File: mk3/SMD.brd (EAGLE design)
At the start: 31.3 x 39 mm, 13 parts, among them IC1 744053D

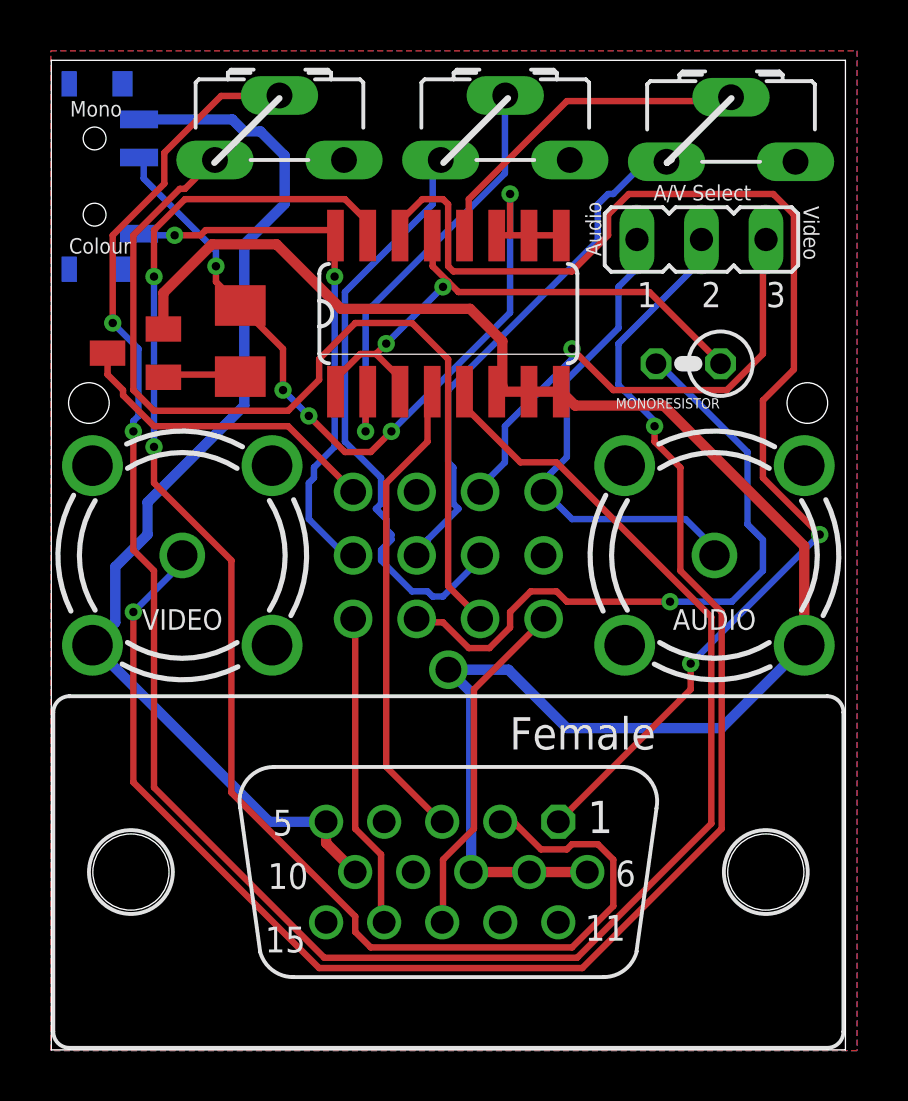
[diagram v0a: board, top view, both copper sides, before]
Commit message: CD4053
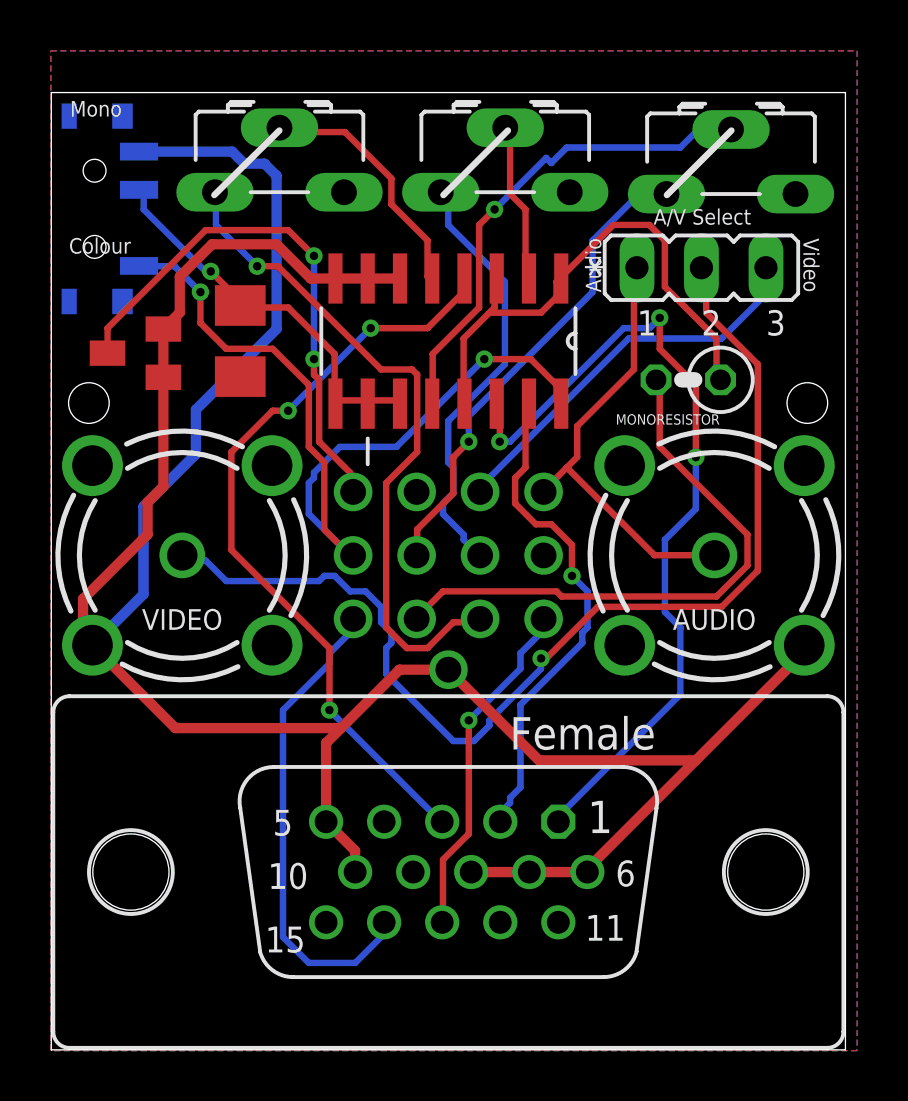
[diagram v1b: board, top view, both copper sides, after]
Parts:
- removed IC1: 744053D, 74xx-eu:SO16
- added U1: CD4053BCM, Fairchild_By_element14_Batch_1:SOIC127P600X175-16N
- moved R7 1.27 mm to (26.8, 33.7)
- moved R8 1.27 mm to (17.9, 33.8)
- moved R9 1.27 mm to (9.00, 33.8)
- moved S1 1.27 mm to (1.72, 33.1)
- moved JP1 1.11 mm to (25.6, 30.8)
- moved MONORESISTOR 0.64 mm to (25.1, 26.4)
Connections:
- removed net N$6: IC1.5, R9.S
- new net N$2: R7.S, U1.12
- net GND: now also U1.6, U1.7, U1.8; no longer IC1.6, IC1.7, IC1.8
- net MONOSIGNAL: now also U1.1, U1.13, U1.3; no longer IC1.1, IC1.13, IC1.3
- net N$4: now also R8.S, U1.2; no longer IC1.12, R7.S
- net N$5: now also R9.S, U1.5; no longer IC1.2, R8.S
- net SELECT: now also U1.10, U1.11, U1.9; no longer IC1.10, IC1.11, IC1.9
- net VBLUE: now also U1.4; no longer IC1.4
- net VCC: now also U1.16; no longer IC1.16
- net VGREEN: now also U1.15; no longer IC1.15
- net VRED: now also U1.14; no longer IC1.14
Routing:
- net N$6: track 80.9 -> 0.00 mm, vias 2 -> 0
- net VGREEN: track 58.9 -> 19.7 mm, vias 2 -> 1
- net N$3: track 64.5 -> 43.5 mm, vias 2 -> 1
- net N$2: track 0.00 -> 19.4 mm, vias 0 -> 1
- net VRED: track 50.7 -> 33.1 mm, vias 2 -> 3
- net SELECT: track 32.7 -> 15.6 mm, vias 5 -> 1
- net VCC: track 21.8 -> 33.6 mm
- net VBLUE: track 18.6 -> 30.3 mm, vias 0 -> 3
- net ABLUE: track 36.5 -> 26.7 mm, vias 0 -> 1
- net MONODETECT: track 12.6 -> 21.1 mm, vias 0 -> 2
- net N$4: track 13.6 -> 6.35 mm
- net N$5: track 17.1 -> 9.90 mm, vias 1 -> 0
- net AGREEN: track 23.7 -> 17.2 mm
- net AVSYNC: track 12.5 -> 19.0 mm
- net GND: track 110.6 -> 104.3 mm
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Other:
- board size 31.3 x 39 mm -> 31.3 x 37.7 mm
